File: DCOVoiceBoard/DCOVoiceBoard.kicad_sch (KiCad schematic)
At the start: 1 part, among them J101 ParentConn

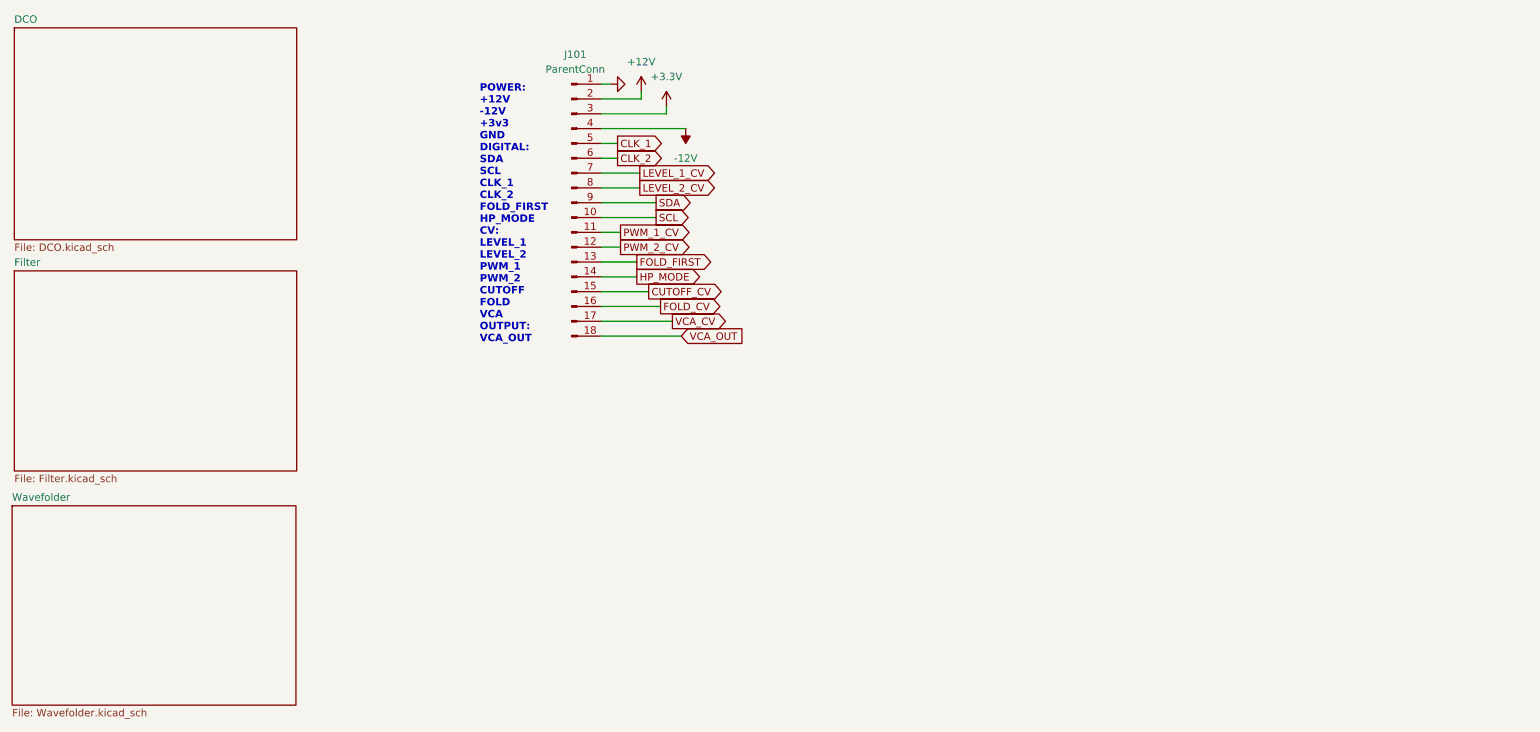
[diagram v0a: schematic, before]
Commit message: motherboard hardware
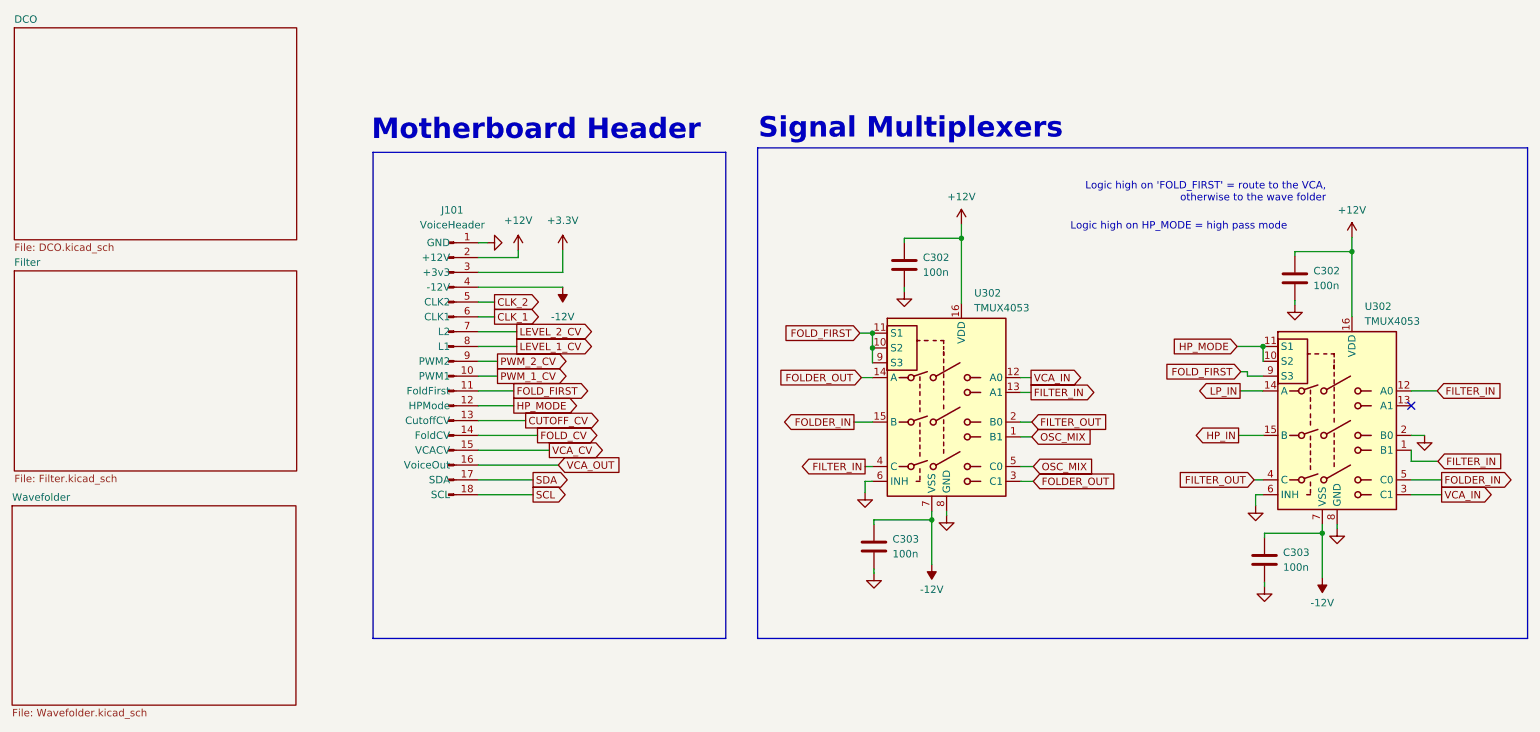
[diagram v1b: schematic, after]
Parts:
- removed J101: ParentConn, Connector_PinHeader_2.54mm:PinHeader_1x18_P2.54mm_Vertical, symbol Connector:Conn_01x18_Pin
- added C302 (x2), C303 (x2): 100n, Capacitor_SMD:C_0805_2012Metric, symbol Device:C
- added J101: VoiceHeader, Connector_PinHeader_2.54mm:PinHeader_1x18_P2.54mm_Vertical, symbol Connector:VoiceBoardConnector_18p
- added U302 (x2): TMUX4053, Package_SO:TSSOP-16_4.4x5mm_P0.65mm, symbol Analog_Switch:TMUX4053
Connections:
- net +12V: now also C302.1, C302.1, J101.2 (+12V), U302.16 (VDD), U302.16 (VDD)
- net +3.3V: now also J101.3 (+3v3)
- net -12V: now also C303.1, C303.1, J101.4 (-12V), U302.7 (VSS), U302.7 (VSS)
- net CLK_1: now also J101.6 (CLK1)
- net CLK_2: now also J101.5 (CLK2)
- net CUTOFF_CV: now also J101.13 (CutoffCV)
- net FOLD_CV: now also J101.14 (FoldCV)
- net FOLD_FIRST: now also J101.11 (FoldFirst), U302.10 (S2), U302.11 (S1), U302.9 (S3), U302.9 (S3)
- net GND: now also C302.2, C302.2, C303.2, C303.2, J101.1 (GND), U302.2 (B0), U302.6 (INH), U302.6 (INH), U302.8 (GND), U302.8 (GND)
- net HP_MODE: now also J101.12 (HPMode), U302.10 (S2), U302.11 (S1)
- net LEVEL_1_CV: now also J101.8 (L1)
- net LEVEL_2_CV: now also J101.7 (L2)
- net PWM_1_CV: now also J101.10 (PWM1)
- net PWM_2_CV: now also J101.9 (PWM2)
- net SCL: now also J101.18 (SCL)
- net SDA: now also J101.17 (SDA)
- net VCA_CV: now also J101.15 (VCACV)
- net VCA_OUT: now also J101.16 (VoiceOut)
- new net FILTER_IN: U302.1 (B1), U302.12 (A0), U302.13 (A1), U302.4 (C)
- new net FILTER_OUT: U302.2 (B0), U302.4 (C)
- new net FOLDER_IN: U302.15 (B), U302.5 (C0)
- new net FOLDER_OUT: U302.14 (A), U302.3 (C1)
- new net HP_IN: U302.15 (B)
- new net LP_IN: U302.14 (A)
- new net OSC_MIX: U302.1 (B1), U302.5 (C0)
- new net VCA_IN: U302.12 (A0), U302.3 (C1)
- no-connect marks 0 -> 1
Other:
- note added: "Logic high on 'FOLD_FIRST' = route to the VCA, otherwise to the wave folder"
- note added: "Logic high on HP_MODE = high pass mode"
- note added: "Motherboard Header"
- note added: "Signal Multiplexers"
- note removed: "POWER: +12V -12V +3v3 GND DIGITAL: SDA SCL CLK_1 CLK_2 FOLD_FIRST HP_MODE CV: LEVEL_1 LEVEL_2 PWM_1 PWM_2 CUTOFF FOLD VCA OUTPUT: VCA_OUT"
